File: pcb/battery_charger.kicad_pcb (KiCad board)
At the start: 2 copper layers, 36.2 x 24.2 mm, 20 parts, among them J1 USB_B_Micro, J2 IN+, J3 IN-, J4 OUT+, J5 BAT+, J6 BAT-, J7 OUT-, U1 TP4056, U2 DW01A, U3 FS8205A

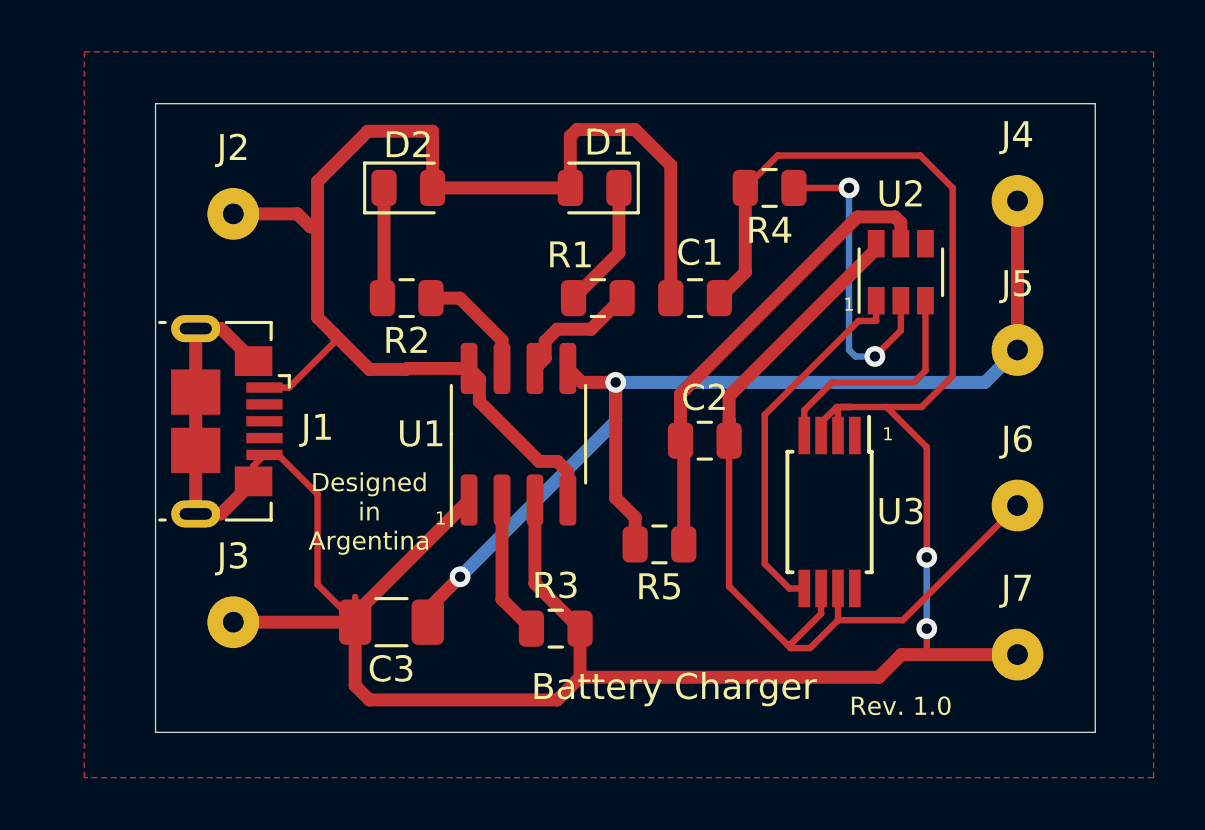
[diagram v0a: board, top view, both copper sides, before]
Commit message: Importantes mejoras en el PCB
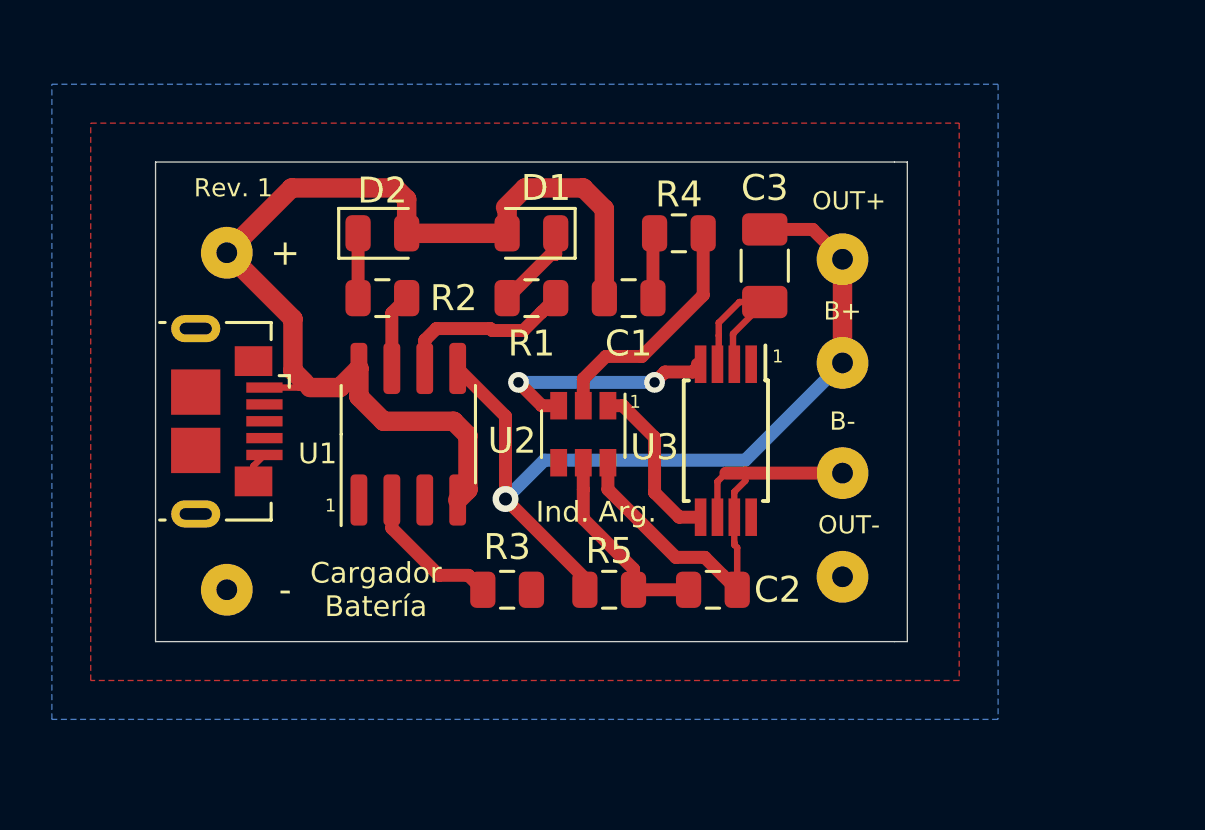
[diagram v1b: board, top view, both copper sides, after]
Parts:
- removed J2: IN+, Connector_Wire:SolderWirePad_1x01_Drill0.8mm
- removed J7: OUT-, Connector_Wire:SolderWirePad_1x01_Drill0.8mm
- added +: IN+, Connector_Wire:SolderWirePad_1x01_Drill0.8mm, F.Cu at (105.2, 123.0)
- added OUT-: OUT-, Connector_Wire:SolderWirePad_1x01_Drill0.8mm, F.Cu at (129.0, 135.5)
- moved C3 19.9 mm to (126.0, 123.5), turned to 270 degrees
- moved U2 13.8 mm to (119.0, 130.0), turned to 270 degrees
- moved OUT+ 7.12 mm to (129.0, 123.2)
- moved B- 6.86 mm to (129.0, 131.5)
- moved B+ 6.77 mm to (129.0, 127.2)
- moved C2 5.76 mm to (124.0, 136.0)
- moved U3 4.85 mm to (124.5, 130.2)
- moved U1 4.25 mm to (112.2, 130.0)
- moved R4 3.91 mm to (122.7, 122.2)
- moved D1 3.00 mm to (117.0, 122.2)
- moved R5 2.61 mm to (120.0, 136.0)
- moved C1 2.56 mm to (120.8, 124.8)
- moved R1 2.56 mm to (117.0, 124.8)
- moved R3 2.40 mm to (116.1, 136.0)
- moved D2 2.02 mm to (111.2, 122.2)
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- renumbered J3 to -, J5 to B+, J6 to B-, J4 to OUT+
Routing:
- net GND: track 109.6 -> 11.4 mm, vias 2 -> 0
- net Net-(C2-Pad2): track 34.0 -> 18.7 mm
- net Net-(C2-Pad1): track 18.1 -> 7.83 mm
- net +5V: track 50.6 -> 41.2 mm
- net Net-(C3-Pad1): track 42.6 -> 33.3 mm, vias 2 -> 1
- net Net-(U2-Pad1): track 14.2 -> 6.48 mm
- net Net-(R4-Pad1): track 12.0 -> 9.38 mm, vias 2 -> 0
- net Net-(R1-Pad2): track 4.87 -> 6.88 mm
- net Net-(D2-Pad1): track 4.28 -> 2.50 mm
- net Net-(D1-Pad1): track 4.97 -> 3.38 mm
- net Net-(R2-Pad1): track 4.50 -> 2.95 mm
- net Net-(U2-Pad3): track 8.98 -> 9.19 mm, vias 0 -> 2
- added copper zone on B.Cu, net GND
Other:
- board size 36.2 x 24.2 mm -> 29 x 18.5 mm
- net class Default: clearance 0.25 -> 0.3
- rule trace_clearance: 0.25 -> 0.3
- board text added: "Cargador Batería"
- board text added: "Grilla componentes: 0.5mm - 0.25mm Grilla pistas: 0.25mm Vías: 1mm Pistas: 0.75mm - 0.5mm - 0.25mm Clearance: 0.3mm (0.2mm para U3) FR4 - 1.6mm espesor Terminación HASL"
- board text added: "Ind. Arg."
- board text added: "Rev. 1"
- board text removed: "Battery Charger"
- board text removed: "Designed in Argentina"
- board text removed: "Rev. 1.0"
